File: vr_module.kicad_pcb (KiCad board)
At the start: 4 copper layers, 20.3 x 22.9 mm, 34 parts, among them J1 Conn_01x07, U1 MAX9142, U2 NC7SB3157P6X, U3 74HC00, U4 NC7SB3157P6X, U5 SRV05-4, U6 MCP6004

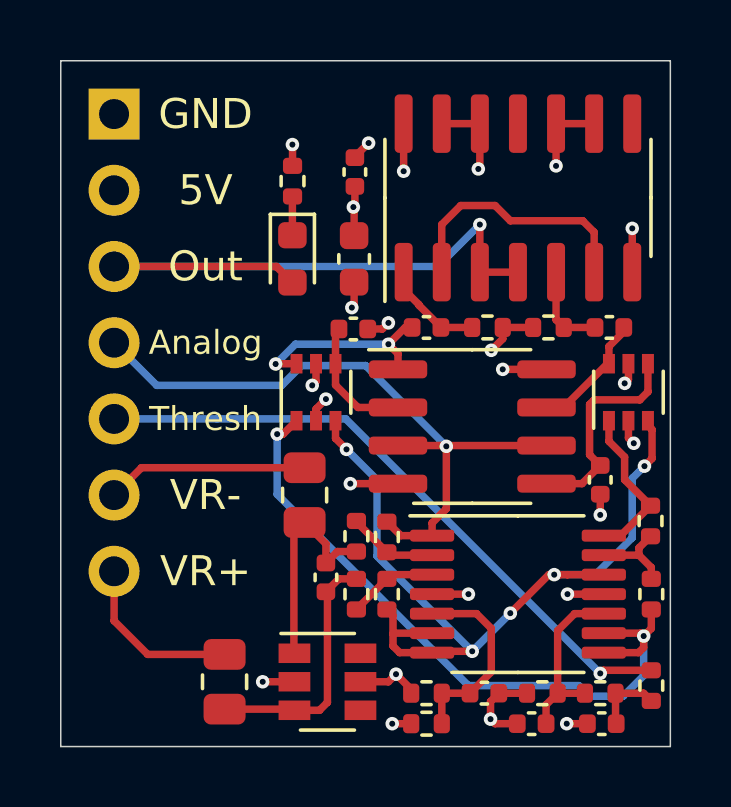
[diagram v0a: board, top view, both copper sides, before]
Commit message: rev b improvements
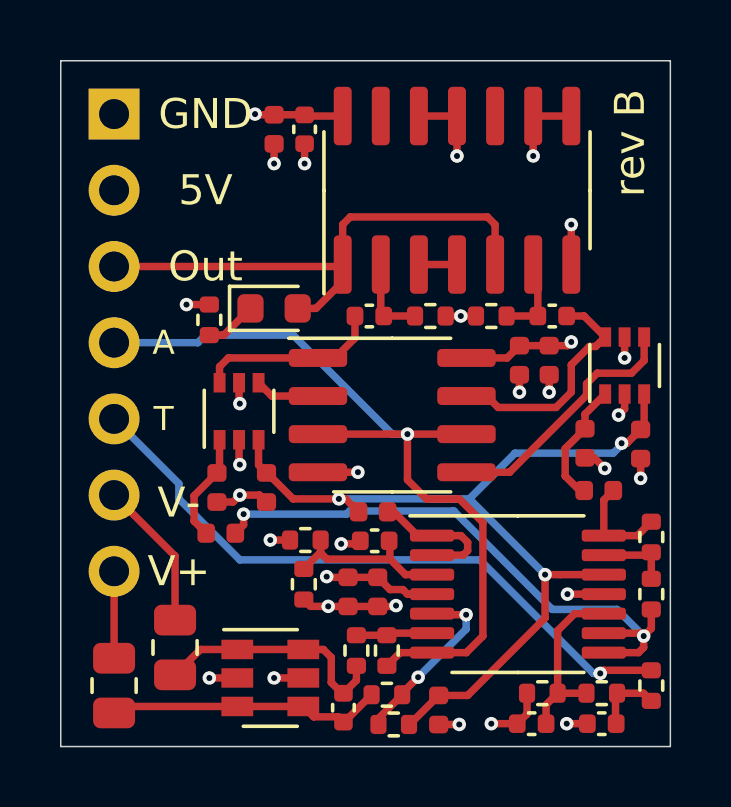
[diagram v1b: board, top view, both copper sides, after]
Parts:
- added C11: 1u, Capacitor_SMD:C_0402_1005Metric, F.Cu at (74.2, 91.0)
- added C12: 1u, Capacitor_SMD:C_0402_1005Metric, F.Cu at (72.3, 91.0)
- added C13: 100n, Capacitor_SMD:C_0402_1005Metric, F.Cu at (67.5, 99.9)
- added C14: 10n, Capacitor_SMD:C_0402_1005Metric, F.Cu at (70.2, 88.2)
- added C15: 1u, Capacitor_SMD:C_0402_1005Metric, F.Cu at (71.1, 88.2)
- added C16: 10n, Capacitor_SMD:C_0402_1005Metric, F.Cu at (65.4, 95.9)
- added C17: 1u, Capacitor_SMD:C_0402_1005Metric, F.Cu at (64.4, 95.9)
- added R17: 10, Resistor_SMD:R_0402_1005Metric, F.Cu at (60.2, 94.0)
- added R18: 10, Resistor_SMD:R_0402_1005Metric, F.Cu at (65.3, 93.3)
- added R19: 10, Resistor_SMD:R_0402_1005Metric, F.Cu at (72.8, 92.6)
- C10, C9: value 10n -> 1u
- C7: footprint Capacitor_SMD:C_0603_1608Metric -> Capacitor_SMD:C_0402_1005Metric
- U3: value 74HC00 -> 74HC02
- moved C10 11.1 mm to (61.7, 92.5), turned to 270 degrees
- moved C9 6.97 mm to (60.1, 92.5), turned to 270 degrees
- moved R7 6.67 mm to (58.7, 97.8)
- moved R9 6.51 mm to (63.0, 94.2)
- moved C4 6.26 mm to (65.3, 94.2), turned to 180 degrees
- moved R10 6.19 mm to (63.0, 95.7), turned to 270 degrees
- moved R16 5.39 mm to (59.8, 86.9)
- moved C7 5.08 mm to (62.0, 80.5)
- moved C5 4.38 mm to (64.3, 99.8)
- moved R5 4.35 mm to (66.0, 100.4), turned to 0 degrees
- moved R3 3.81 mm to (64.7, 97.9)
- moved R6 3.78 mm to (65.7, 97.9), turned to 90 degrees
- moved R8 3.69 mm to (56.6, 99.1)
- moved R4 3.50 mm to (65.7, 99.4), turned to 0 degrees
- moved U1 2.69 mm to (65.9, 90.0)
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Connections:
- C10 pad 1: GND -> Vref
- C10 pad 2: Net-(C10-Pad2) -> GND
- C9 pad 1: GND -> thresh_low
- C9 pad 2: Net-(C9-Pad2) -> GND
- R11 pad 1: Net-(C8-Pad1) -> Net-(C3-Pad1)
- R11 pad 2: Net-(C3-Pad1) -> Net-(C8-Pad1)
- R13 pad 2: thresh_low -> Net-(R13-Pad2)
- R14 pad 1: thresh_high -> Net-(R14-Pad1)
- U1 pad 2: Net-(C9-Pad2) -> Net-(U1-Pad2)
- U1 pad 5: Net-(C10-Pad2) -> Net-(U1-Pad5)
- U2 pad 4: Net-(C9-Pad2) -> Net-(U1-Pad2)
- U3 pad 1: Net-(C1-Pad1) -> output
- U3 pad 10: GND -> (no net)
- U3 pad 11: (no net) -> GND
- U3 pad 13: GND -> (no net)
- U3 pad 2: Net-(U3-Pad2) -> Net-(C1-Pad1)
- U3 pad 3: output -> Net-(U3-Pad3)
- U3 pad 4: output -> Net-(U3-Pad3)
- U3 pad 5: Net-(C2-Pad1) -> output
- U3 pad 6: Net-(U3-Pad2) -> Net-(C2-Pad1)
- U3 pad 8: (no net) -> GND
- U4 pad 4: Net-(C10-Pad2) -> Net-(U1-Pad5)
- U5 pad 4: (no net) -> Net-(C5-Pad2)
- U5 pad 6: (no net) -> Net-(C5-Pad1)
- U6 pad 1: analog_out -> Net-(R18-Pad1)
- U6 pad 14: thresh_high -> Net-(R14-Pad1)
- U6 pad 2: Net-(R3-Pad1) -> Net-(R18-Pad1)
- U6 pad 3: Net-(R4-Pad2) -> Net-(C4-Pad1)
- U6 pad 5: Net-(C4-Pad1) -> Net-(R4-Pad2)
- U6 pad 6: Vref -> Net-(R3-Pad1)
- U6 pad 7: Vref -> analog_out
- U6 pad 8: thresh_low -> Net-(R13-Pad2)
- U6 pad 9: thresh_low -> Net-(R13-Pad2)
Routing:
- net Net-(R13-Pad2): track 0.00 -> 20.0 mm, vias 0 -> 2
- net thresh_low: track 23.6 -> 3.63 mm, vias 2 -> 0
- net Net-(U3-Pad2): track 8.63 -> 0.00 mm
- net Net-(U1-Pad5): track 0.00 -> 8.47 mm
- net Net-(C10-Pad2): track 7.28 -> 0.00 mm
- net Net-(R18-Pad1): track 0.00 -> 4.61 mm
- net Net-(C9-Pad2): track 4.31 -> 0.00 mm
- net GND: track 22.3 -> 26.5 mm, vias 17 -> 23
- net +5V: track 9.55 -> 13.5 mm
- net analog_out: track 24.3 -> 28.2 mm
- net Net-(C2-Pad2): track 4.10 -> 7.86 mm
- net output: track 21.8 -> 18.0 mm, vias 1 -> 0
- net Net-(R14-Pad1): track 0.00 -> 3.41 mm
- net Net-(R4-Pad2): track 3.01 -> 6.02 mm, vias 0 -> 2
- net VR+: track 5.80 -> 2.90 mm
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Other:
- board text added: "A"
- board text added: "T"
- board text added: "V+"
- board text added: "V-"
- board text added: "rev B"
- board text removed: "Analog"
- board text removed: "Thresh"
- board text removed: "VR+"
- board text removed: "VR-"
